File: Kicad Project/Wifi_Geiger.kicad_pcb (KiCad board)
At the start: 2 copper layers, 100 x 25 mm, 49 parts, among them J1 USB_B_Mini, J2 Conn_01x04, Q1 MMBTA42LT1G, Q2 MMBT3904-TP, Q3 MMBT3904-TP, U1 NE555DR, U2 MIC5504-3.3YM5, U3 NE555DR, U4 LM2904, U5 ESP-12E

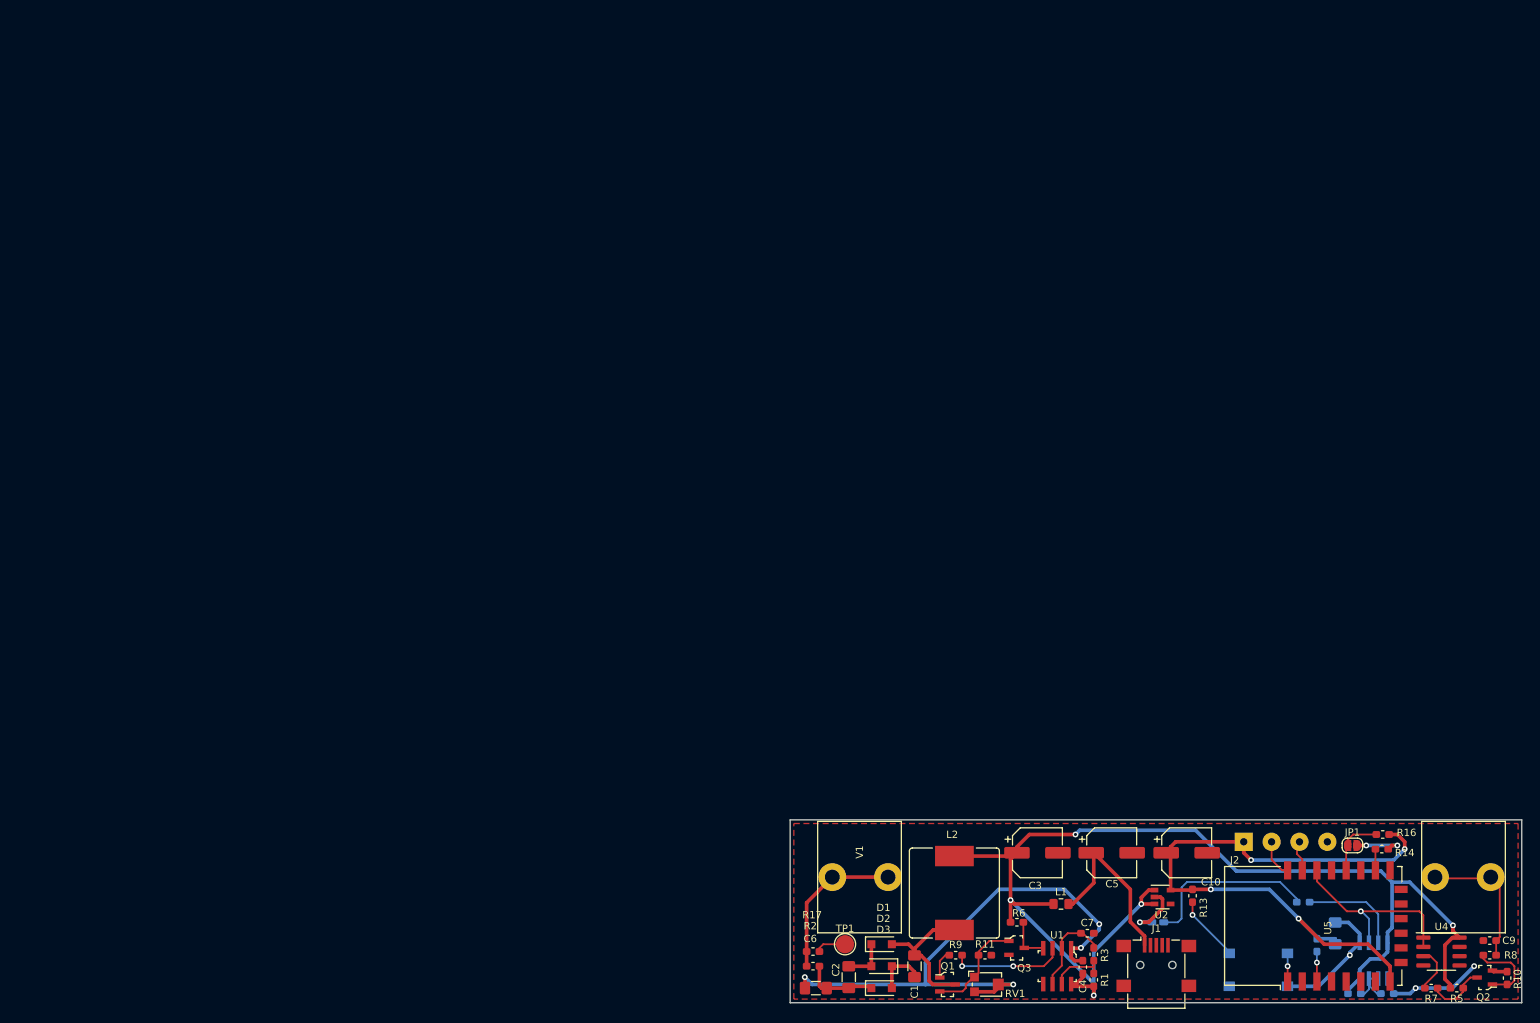
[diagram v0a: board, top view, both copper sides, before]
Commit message: Final commit for video
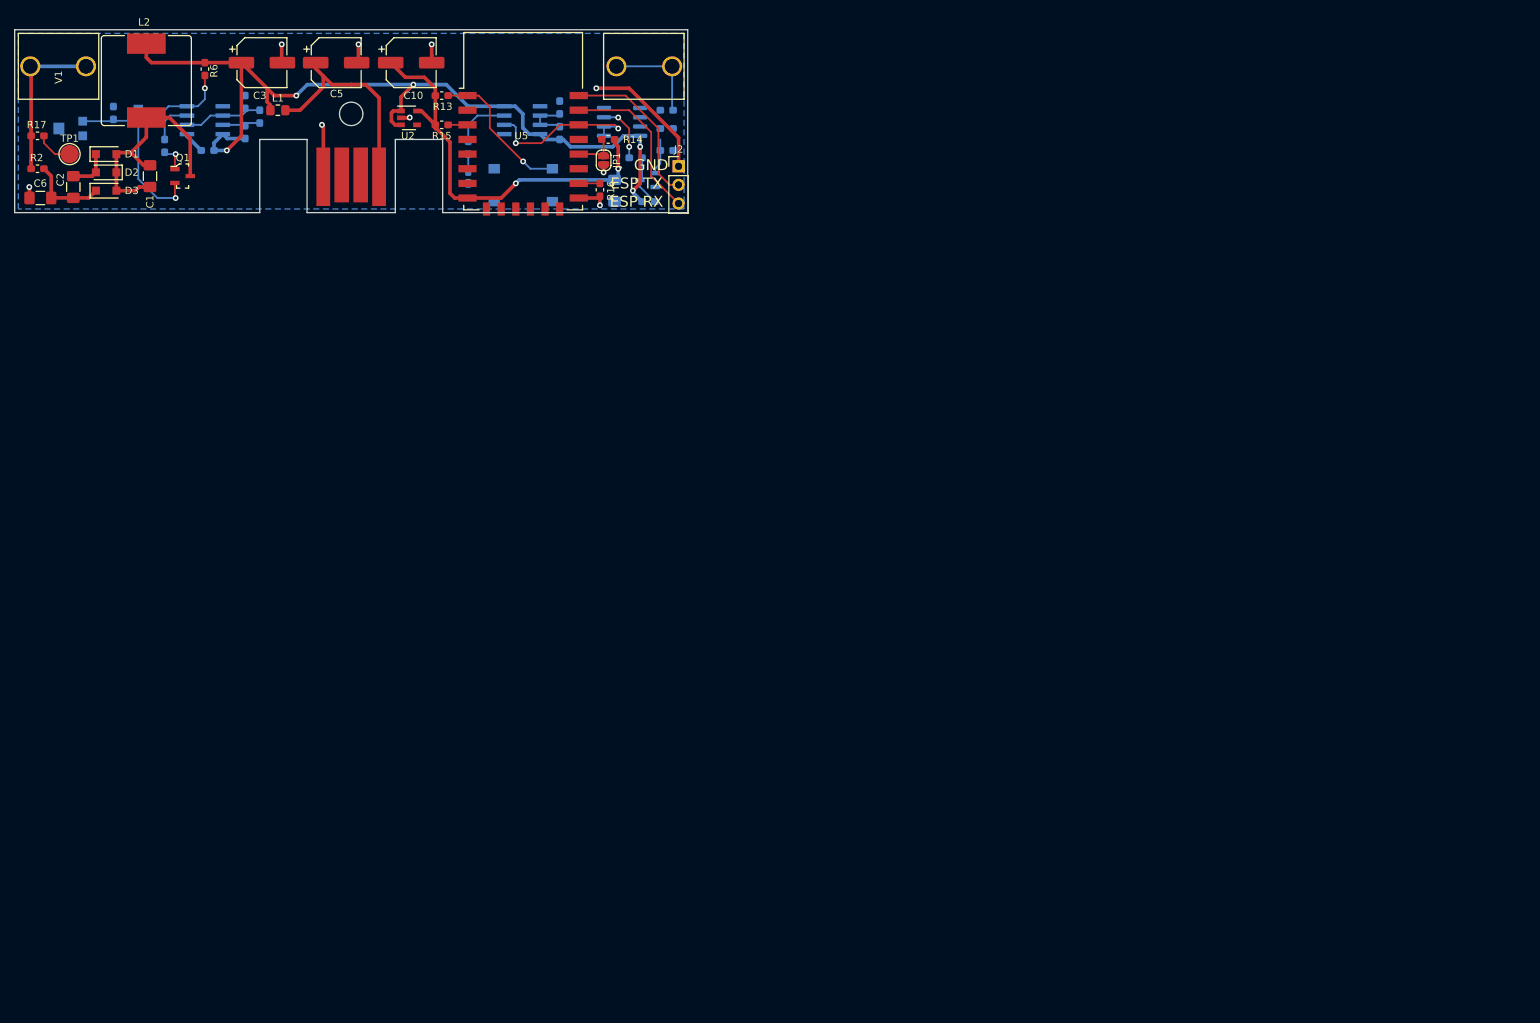
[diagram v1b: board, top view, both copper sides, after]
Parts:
- added REF**: MountingHole_3.2mm_M3, MountingHole:MountingHole_3.2mm_M3, F.Cu at (46.0, 11.5)
- C4, C7, C9, Q2, Q3, R1, R10, R11, R3, R5, R7, R8, R9, RV1, U1, U4: moved to B.Cu
- J1: value USB_B_Mini -> 4_PIN_USB; footprint Connector_USB:USB_Mini-B_Lumberg_2486_01_Horizontal -> usb_traces:usb-traces
- J2: value Conn_01x04 -> Conn_01x03_Male; footprint Connector_Wire:SolderWirePad_1x04_P3.81mm_Drill1mm -> Connector_PinHeader_2.54mm:PinHeader_1x03_P2.54mm_Vertical
- R15: moved to F.Cu
- moved RV1 171.6 mm to (7.50, 13.5), turned to 180 degrees
- moved C8 165.7 mm to (74.5, 10.6), turned to 90 degrees
- moved R11 165.7 mm to (13.5, 11.4), turned to 270 degrees
- moved Q3 164.8 mm to (17.9, 11.5)
- moved U1 164.1 mm to (26.0, 12.4), turned to 90 degrees
- moved R1 164.0 mm to (31.5, 14.0)
- moved R15 164.0 mm to (58.4, 13.0), turned to 0 degrees
- moved C4 163.6 mm to (26.4, 16.5), turned to 180 degrees
- moved U3 163.5 mm to (69.4, 12.4), turned to 90 degrees
- moved C7 161.8 mm to (31.5, 9.88), turned to 90 degrees
- moved R3 161.6 mm to (33.5, 11.9)
- moved R10 161.2 mm to (89.1, 16.5), turned to 180 degrees
- moved R6 161.0 mm to (26.0, 5.38), turned to 90 degrees
- moved R4 160.1 mm to (74.5, 14.1), turned to 90 degrees
- moved C9 159.8 mm to (89.1, 11.0)
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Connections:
- J1 pad 4: Net-(J1-Pad4) -> GND
- J2 pad 1: +3V3 -> GND
- S1 pad 3: Net-(R13-Pad1) -> Net-(S1-Pad3)
- S1 pad 4: Net-(S1-Pad4) -> Net-(R13-Pad1)
- U5 pad 1: Net-(S1-Pad4) -> Net-(R13-Pad1)
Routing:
- net GND: track 125.3 -> 44.0 mm, vias 10 -> 9
- net +5V: track 165.4 -> 119.5 mm
- net +3V3: track 89.1 -> 56.1 mm, vias 4 -> 2
- net Net-(D4-Pad2): track 24.4 -> 2.38 mm
- net /ESP_RXD: track 4.40 -> 22.4 mm
- net /ESP_TXD: track 5.25 -> 22.3 mm
- net Net-(R13-Pad1): track 9.08 -> 20.1 mm
- net /555_SQUARE_WAVE: track 15.6 -> 5.87 mm, vias 2 -> 0
- net Net-(Q1-Pad2): track 14.3 -> 24.0 mm, vias 0 -> 1
- net Net-(R12-Pad2): track 14.0 -> 7.69 mm
- net /5V_RAW: track 24.3 -> 29.9 mm
- net Net-(Q2-Pad1): track 10.3 -> 4.89 mm
- net /555_FEEDBACK: track 6.17 -> 11.1 mm, vias 0 -> 1
- net Net-(C9-Pad2): track 18.3 -> 13.7 mm
- net /GEIGER_PULSE: track 27.1 -> 22.5 mm, vias 1 -> 2
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- added copper zone on B.Cu, net GND
- removed copper zone on F.Cu, net GND
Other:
- board size 100 x 25 mm -> 92 x 25 mm
- board text added: "ESP RX"
- board text added: "ESP TX"
- board text added: "GND"
